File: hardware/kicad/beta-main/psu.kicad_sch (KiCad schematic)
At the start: 0 parts

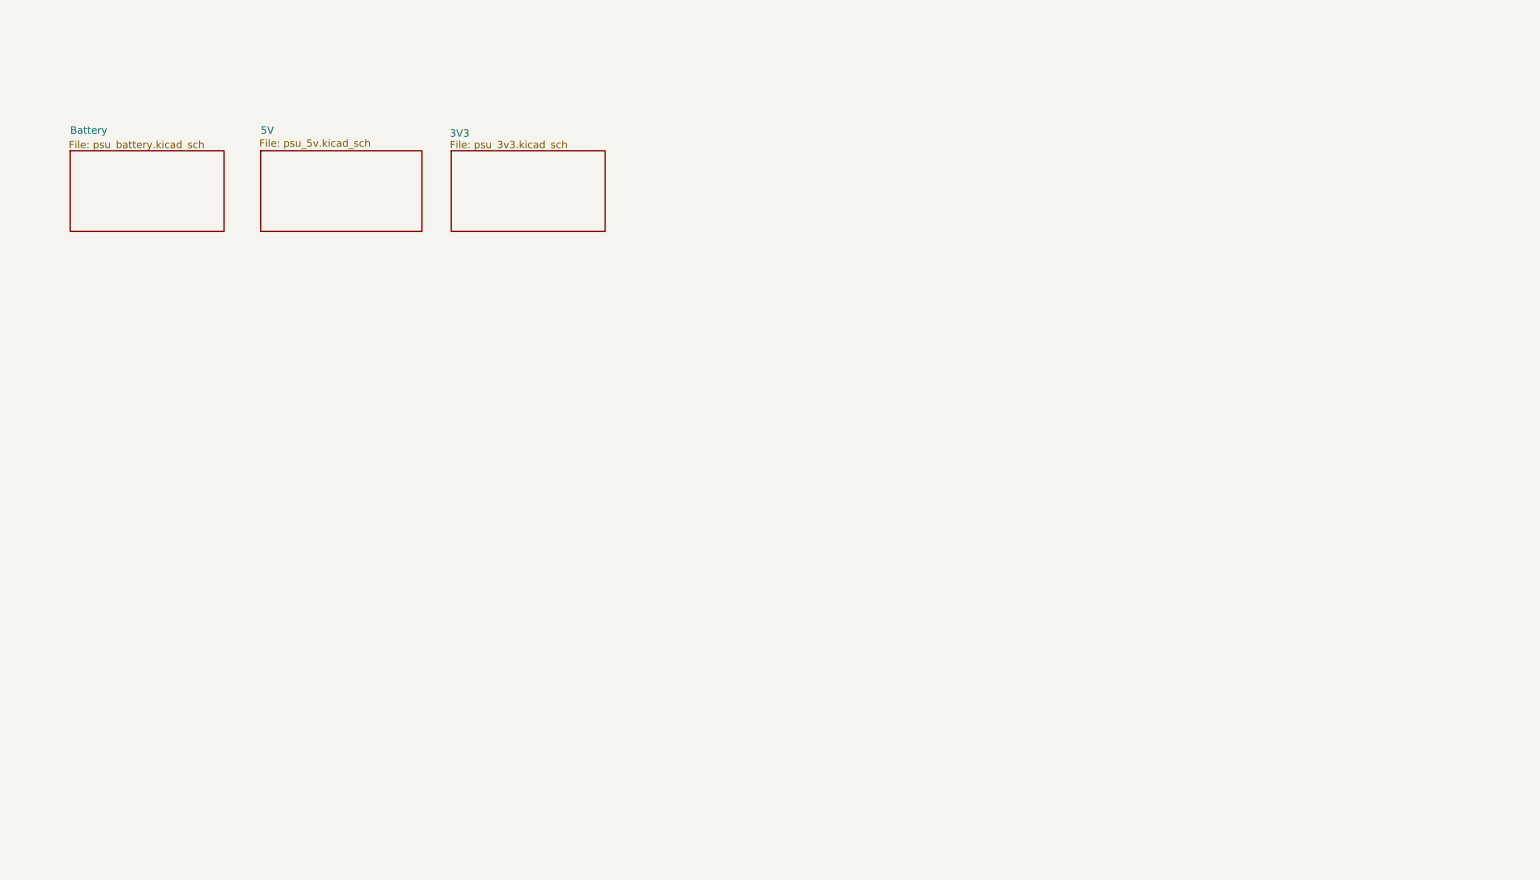
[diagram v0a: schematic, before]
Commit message: add modifications
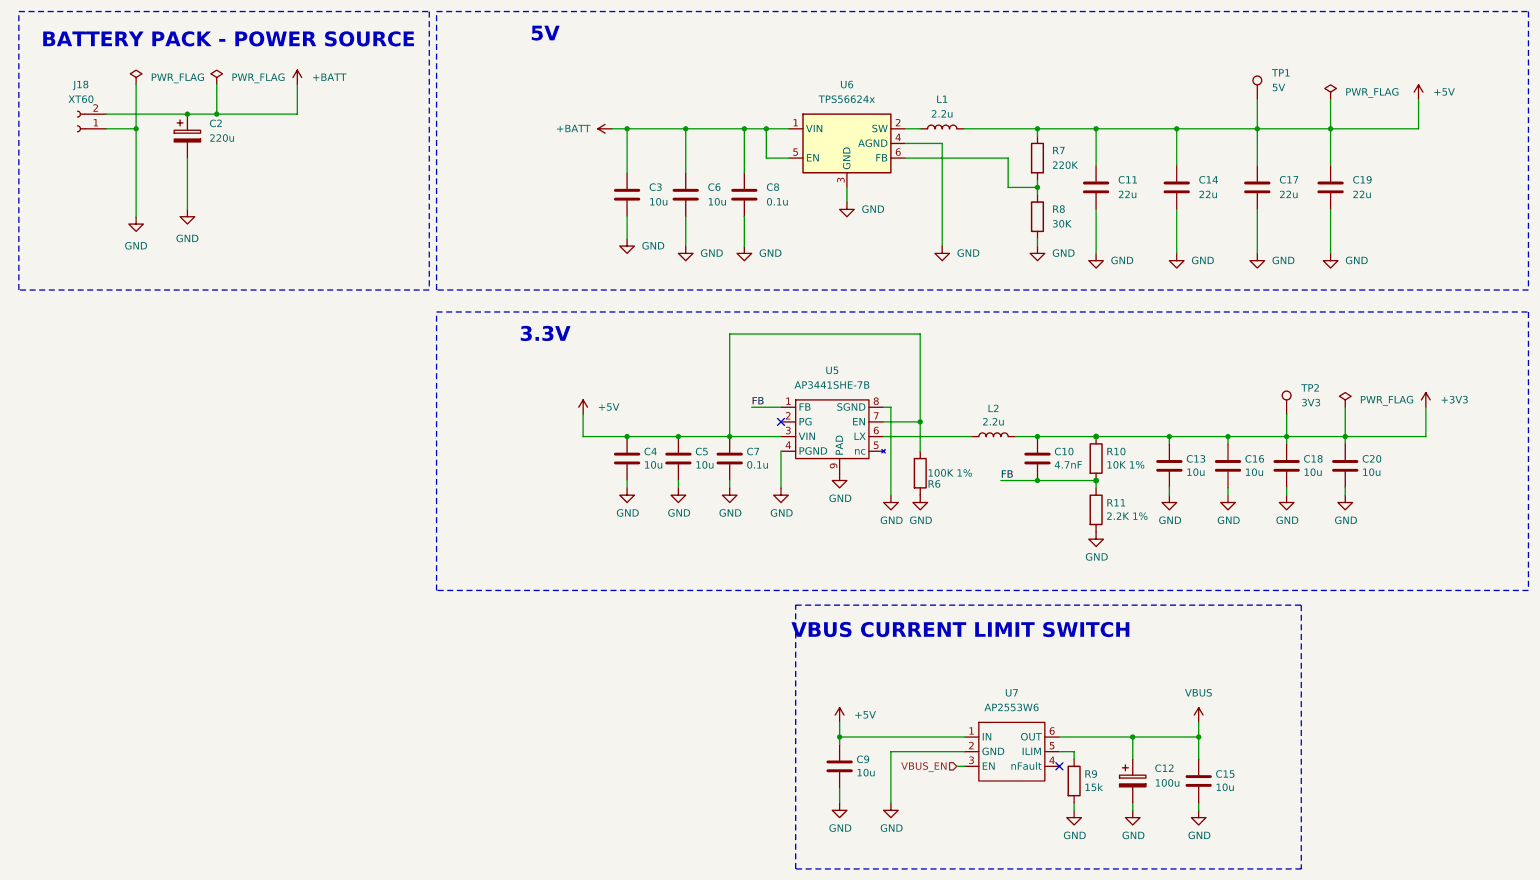
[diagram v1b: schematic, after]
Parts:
- added C10: 4.7nF, Capacitor_SMD:C_0402_1005Metric, symbol Device:C
- added C11, C14, C17, C19: 22u, Capacitor_SMD:C_0603_1608Metric_Pad1.08x0.95mm_HandSolder, symbol Device:C
- added C12: 100u, Capacitor_SMD:C_0603_1608Metric_Pad1.08x0.95mm_HandSolder, symbol Device:C_Polarized
- added C13, C15, C16, C18, C20, C3, C4, C5, C6, C9: 10u, Capacitor_SMD:C_0603_1608Metric_Pad1.08x0.95mm_HandSolder, symbol Device:C
- added C2: 220u, Capacitor_SMD:C_0603_1608Metric_Pad1.08x0.95mm_HandSolder, symbol Device:C_Polarized
- added C7, C8: 0.1u, Capacitor_SMD:C_0402_1005Metric, symbol Device:C
- added J18: XT60, Connector_AMASS:AMASS_XT60-F_1x02_P7.20mm_Vertical, symbol Connector:Conn_01x02_Socket
- added L1, L2: 2.2u, CM5IO:L_Bourns_SRP5030CC, symbol Device:L
- added R10: 10K 1%, Resistor_SMD:R_0402_1005Metric, symbol Device:R
- added R11: 2.2K 1%, Resistor_SMD:R_0402_1005Metric, symbol Device:R
- added R6: 100K 1%, Resistor_SMD:R_0402_1005Metric, symbol Device:R
- added R7: 220K, Resistor_SMD:R_0402_1005Metric, symbol Device:R
- added R8: 30K, Resistor_SMD:R_0402_1005Metric, symbol Device:R
- added R9: 15k, Resistor_SMD:R_0402_1005Metric, symbol Device:R
- added TP1: 5V, TestPoint:TestPoint_Pad_D1.0mm, symbol Connector:TestPoint
- added TP2: 3V3, TestPoint:TestPoint_Pad_D1.0mm, symbol Connector:TestPoint
- added U5: AP3441SHE-7B, Package_DFN_QFN:DFN-8-1EP_2x2mm_P0.5mm_EP1.05x1.75mm, symbol CM5IO:AP3441SHE-7B
- added U6: TPS56624x, Package_TO_SOT_SMD:SOT-563, symbol Beta:TPS56624x
- added U7: AP2553W6, Package_TO_SOT_SMD:SOT-23-6, symbol CM5IO:AP2553W6
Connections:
- new net: R7.2, R8.1, U6.6 (FB)
- new net: L1.1, U6.2 (SW)
- new net: R9.1, U7.5 (ILIM)
- new net: L2.1, U5.6 (LX)
- new net +3V3: C10.1, C13.1, C16.1, C18.1, C20.1, L2.2, R10.1, TP2.1
- new net +5V: C11.1, C14.1, C17.1, C19.1, C4.1, C5.1, C7.1, C9.1, L1.2, R6.1, R7.1, TP1.1, U5.3 (VIN), U5.7 (EN), U7.1 (IN)
- new net +BATT: C2.1, C3.1, C6.1, C8.1, J18.2 (Pin_2), U6.1 (VIN), U6.5 (EN)
- new net FB: C10.2, R10.2, R11.1, U5.1 (FB)
- new net GND: C11.2, C12.2, C13.2, C14.2, C15.2, C16.2, C17.2, C18.2, C19.2, C2.2, C20.2, C3.2, C4.2, C5.2, C6.2, C7.2, C8.2, C9.2, J18.1 (Pin_1), R11.2, R6.2, R8.2, R9.2, U5.4 (PGND), U5.8 (SGND), U5.9 (PAD), U6.3 (GND), U6.4 (AGND), U7.2 (GND)
- new net VBUS: C12.1, C15.1, U7.6 (OUT)
- new net VBUS_EN: U7.3 (EN)
- no-connect marks 0 -> 2
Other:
- removed sheet 3V3
- removed sheet 5V
- removed sheet Battery
- note added: "3.3V"
- note added: "5V"
- note added: "BATTERY PACK - POWER SOURCE"
- note added: "VBUS CURRENT LIMIT SWITCH"
